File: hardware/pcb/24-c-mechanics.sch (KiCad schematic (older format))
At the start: 22 parts, among them U301 VID28-05, U302 VID66-08, U303 AH3572, U304 AH3572

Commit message: Included all 3D files
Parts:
- U303, U304: footprint Package_TO_SOT_SMD:SOT-23 -> mvl-footprints:SOT-23-UD
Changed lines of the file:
@@
 F 0 "U303" H 5670 5096 50  0000 R CNN
 F 1 "AH3572" H 5670 5005 50  0000 R CNN
-F 2 "Package_TO_SOT_SMD:SOT-23" H 5950 5050 50  0001 C CNN
+F 2 "mvl-footprints:SOT-23-UD" H 5950 5050 50  0001 C CNN
 F 3 "https://www.diodes.com/assets/Datasheets/AH3572.pdf" H 5950 5050 50  0001 C CNN
 F 4 "-MASTER" H 6000 5050 50  0001 C CNN "Config"
@@
 F 0 "U304" H 7870 5096 50  0000 R CNN
 F 1 "AH3572" H 7870 5005 50  0000 R CNN
-F 2 "Package_TO_SOT_SMD:SOT-23" H 8150 5050 50  0001 C CNN
+F 2 "mvl-footprints:SOT-23-UD" H 8150 5050 50  0001 C CNN
 F 3 "https://www.diodes.com/assets/Datasheets/AH3572.pdf" H 8150 5050 50  0001 C CNN
 F 4 "-MASTER" H 8200 5050 50  0001 C CNN "Config"

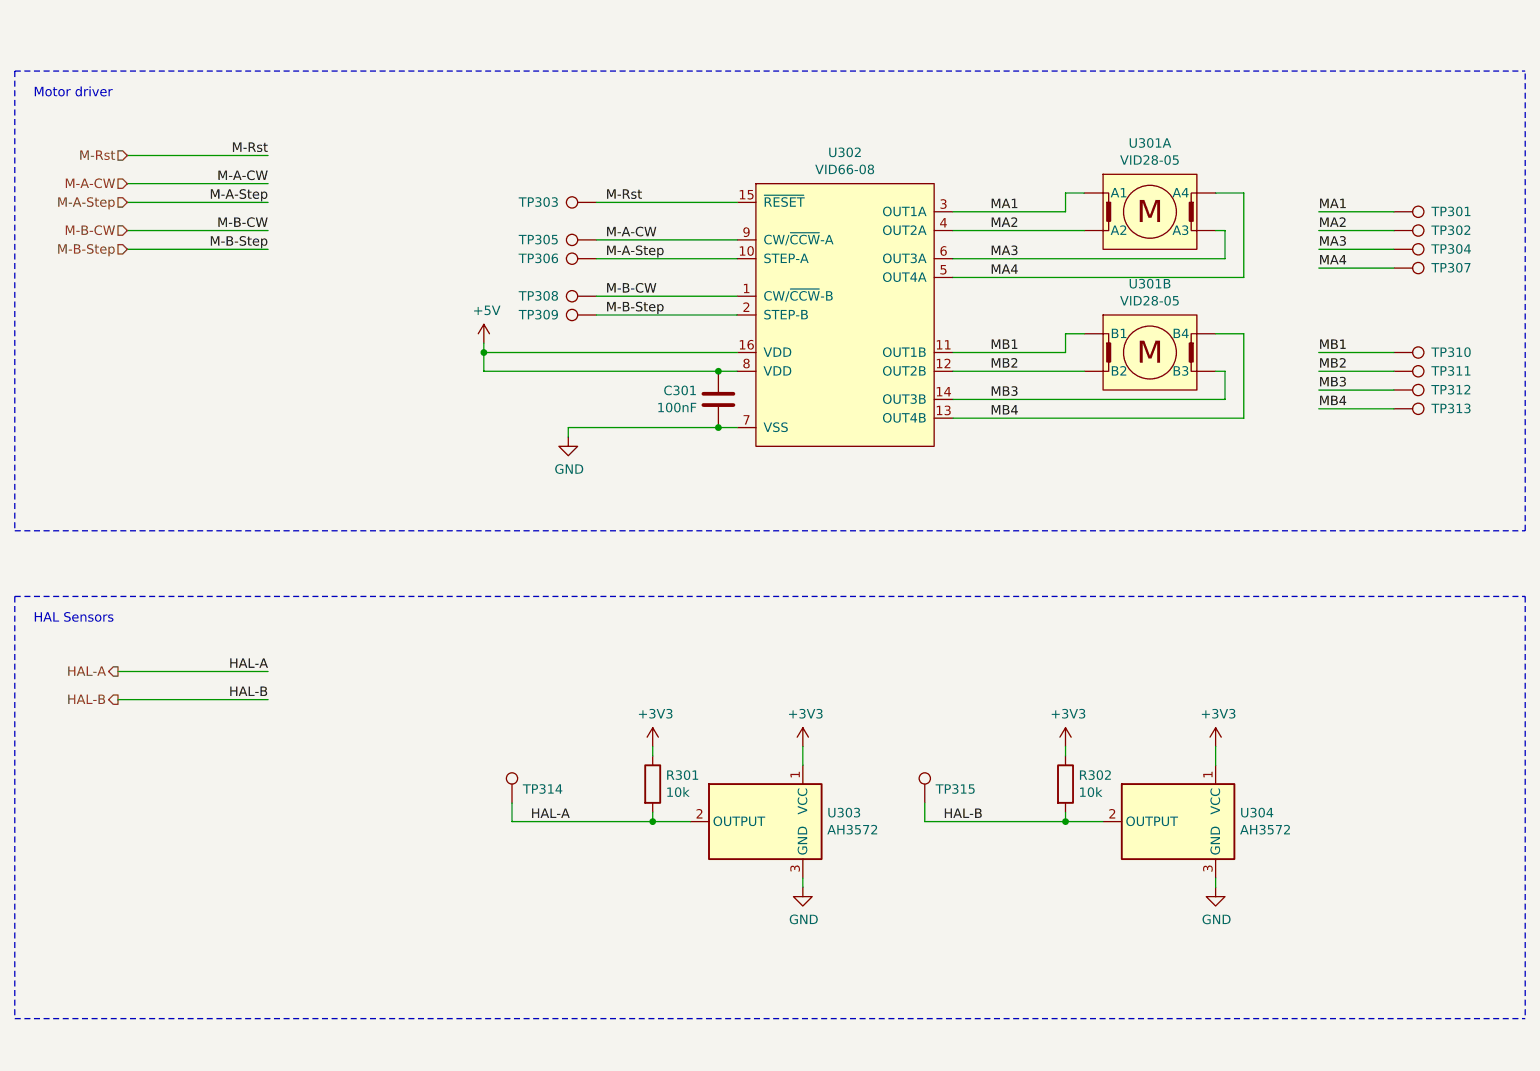
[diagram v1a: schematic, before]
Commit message: Mixed changes
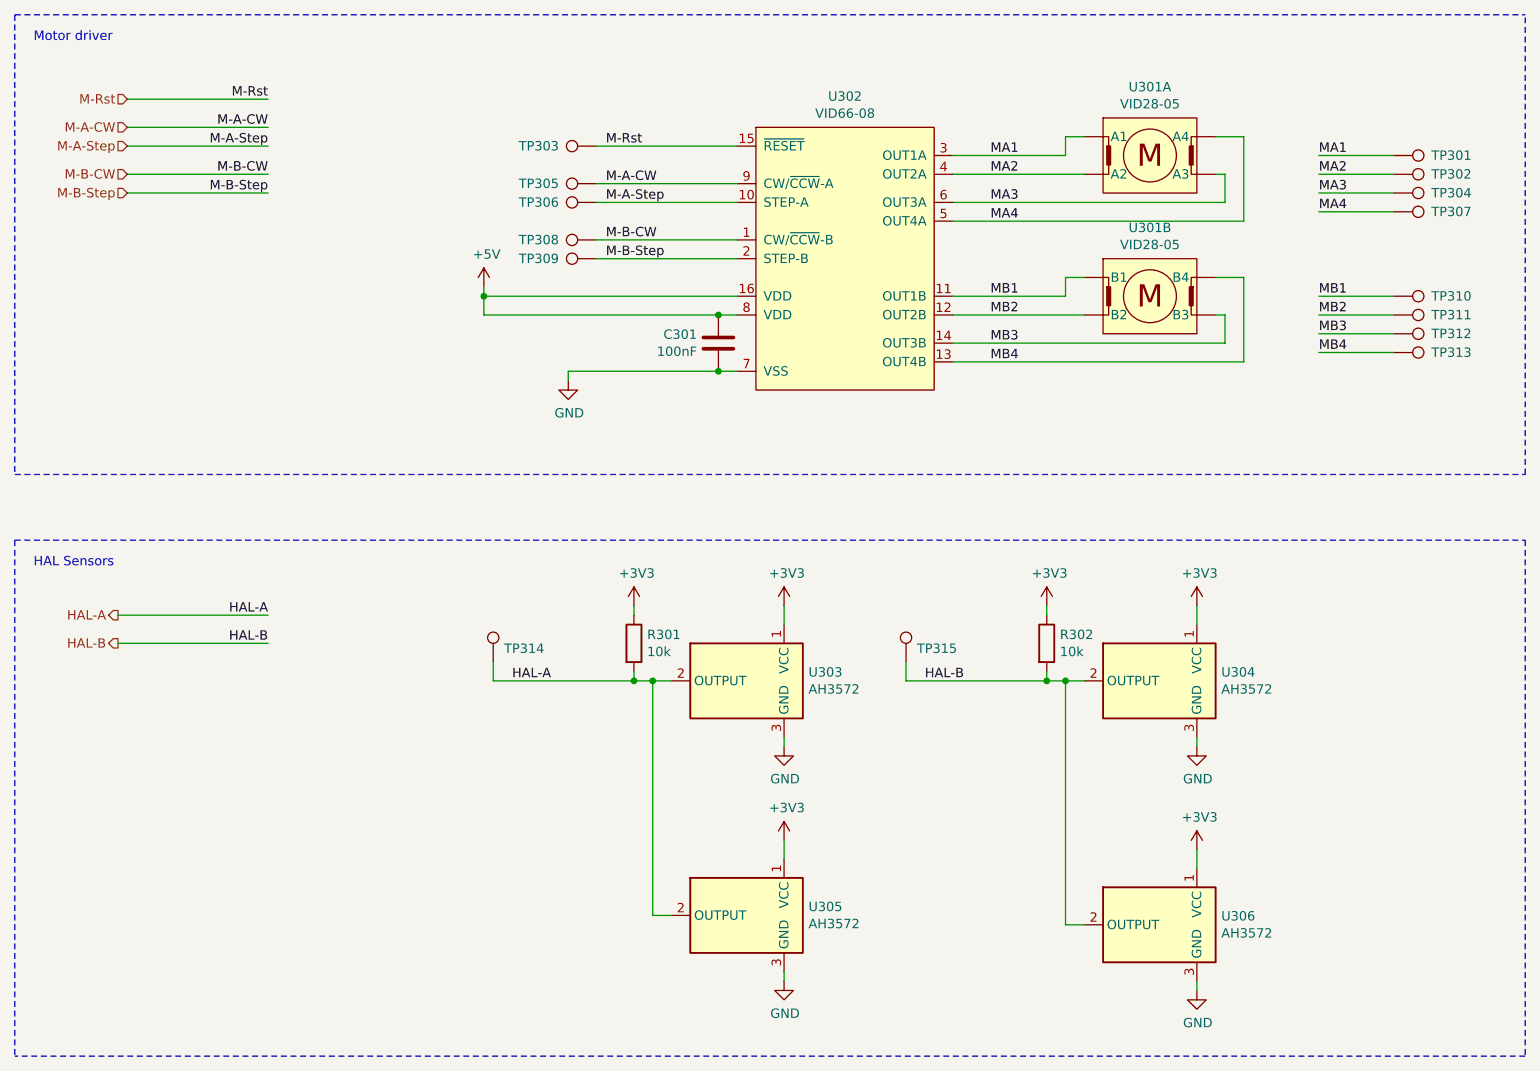
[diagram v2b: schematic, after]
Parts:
- added U305, U306: AH3572, Package_TO_SOT_SMD:TSOT-23, symbol Sensor_Magnetic:SM351LT
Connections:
- net +3V3: now also U305.1 (VCC), U306.1 (VCC)
- net GND: now also U305.3 (GND), U306.3 (GND)
- net HAL-A: now also U305.2 (OUTPUT)
- net HAL-B: now also U306.2 (OUTPUT)
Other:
- moved on the sheet: C301, R301, R302, TP301, TP302, TP303, TP304, TP305, TP306, TP307, TP308, TP309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
